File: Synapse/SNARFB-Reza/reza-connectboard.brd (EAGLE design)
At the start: 100 x 80 mm, 6 parts

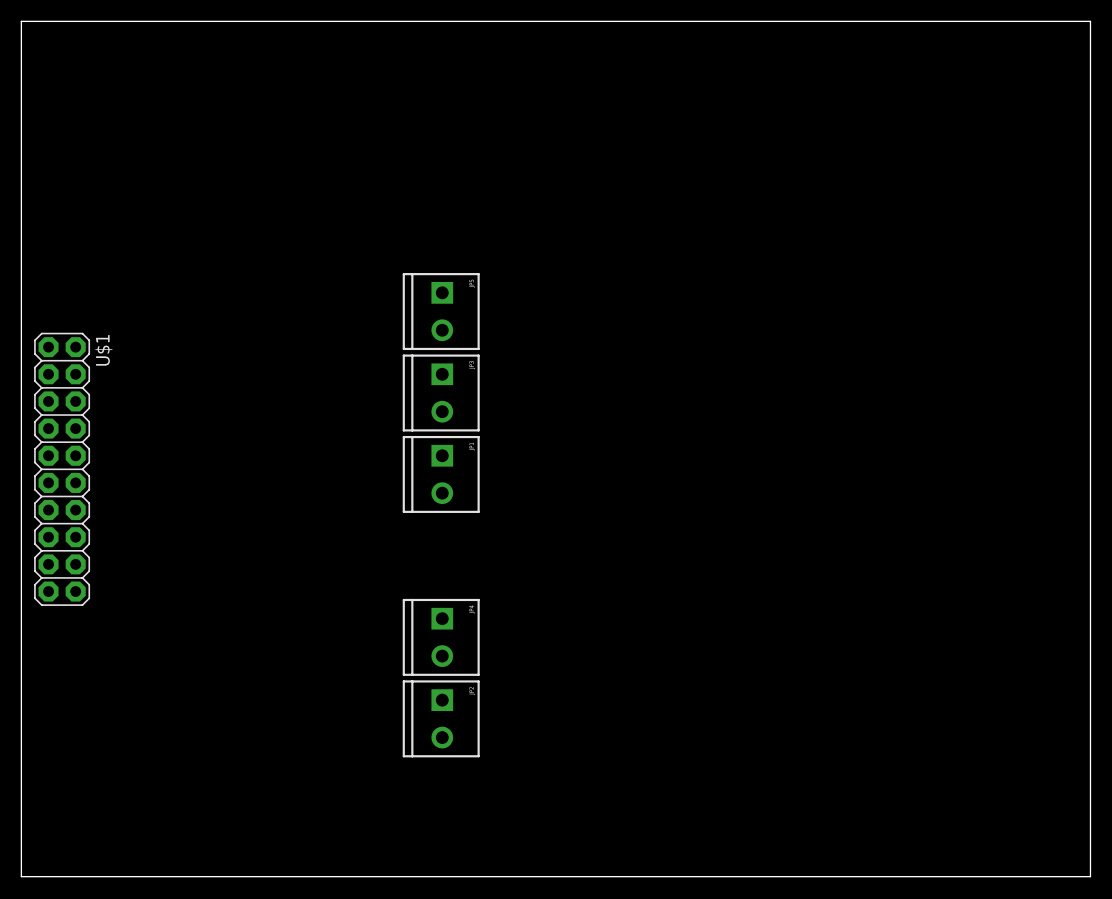
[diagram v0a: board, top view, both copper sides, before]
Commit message: sync
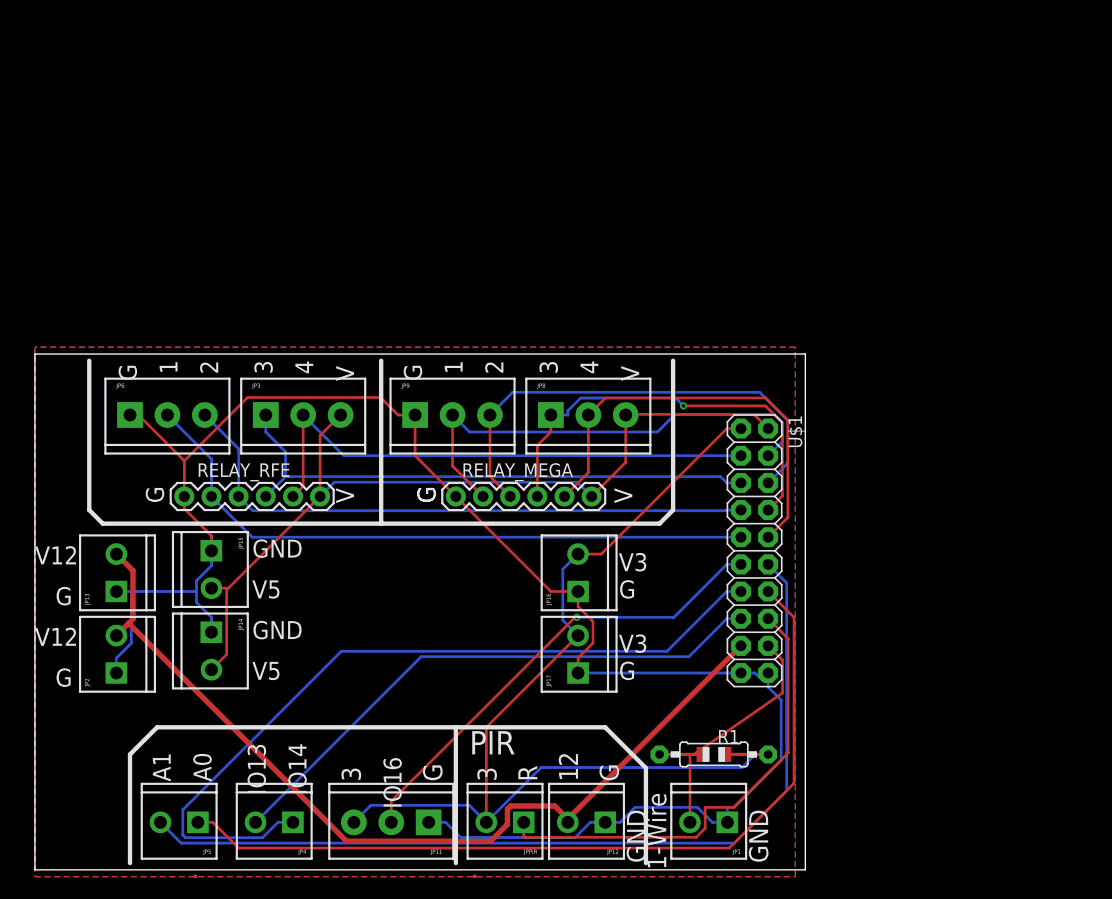
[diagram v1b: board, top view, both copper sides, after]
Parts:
- added JP11, JP6, JP8, JP9: (no value), SparkFun-Connectors:SCREWTERMINAL-3.5MM-3
- added JP12, JP13, JP14, JP15, JP16, JP17, JPPIR: M023.5MM, SparkFun-Connectors:SCREWTERMINAL-3.5MM-2
- added R1: (no value), adafruit:0805-THM
- added RELAY_MEGA, RELAY_RFE: (no value), SparkFun-Connectors:1X06
- added U$2: (no value), 0_jc-custom-eagle6:ENVIOSYS_LOGO2
- JP3: value M023.5MM -> (none); device SparkFun-Connectors:SCREWTERMINAL-3.5MM-2 -> SparkFun-Connectors:SCREWTERMINAL-3.5MM-3
- moved U$1 65.2 mm to (68.6, 30.5)
- moved JP5 54.6 mm to (16.5, 5.08), turned to 180 degrees
- moved JP1 43.4 mm to (66.0, 5.08), turned to 180 degrees
- moved JP2 30.6 mm to (8.89, 19.1), turned to 90 degrees
- moved JP4 23.6 mm to (25.4, 5.08), turned to 180 degrees
- moved JP3 16.9 mm to (22.9, 43.2), turned to 0 degrees
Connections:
- net GND: now also JP1.1, JP11.1, JP12.1, JP13.1, JP14.1, JP15.1, JP16.1, JP17.1, JP2.1, JP6.1, JP9.1, RELAY_MEGA.1, RELAY_RFE.1
- net GPIO13: now also JP4.2
- net GPIO14: now also JP4.1
- net GPIO15: now also JP6.2, RELAY_RFE.2
- net GPIO16: now also JP11.2
- net GPIO2: now also JP3.2, RELAY_RFE.5
- net GPIO5: now also JP3.1, RELAY_RFE.4
- net GPIO6: now also JP6.3, RELAY_RFE.3
- net PC6-D5: now also JPPIR.1
- net PD7-D6: now also JP1.2, R1.2
- net PF0-A5: now also JP9.2, RELAY_MEGA.2
- net PF1-A4: now also JP9.3, RELAY_MEGA.3
- net PF4-A3: now also JP8.1, RELAY_MEGA.4
- net PF5-A2: now also JP8.2, RELAY_MEGA.5
- net PF6-A1: now also JP5.2
- net PF7-A0: now also JP5.1
- net VCC12: now also JP12.2, JP13.2, JP2.2
- net VCC3: now also JP11.3, JP16.2, JP17.2, JPPIR.2, R1.1
- net VCC5: now also JP14.2, JP15.2, JP3.3, JP8.3, RELAY_MEGA.6, RELAY_RFE.6
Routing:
- net GND: track 0.00 -> 163.8 mm
- net VCC3: track 0.00 -> 92.6 mm
- net VCC12: track 0.00 -> 84.3 mm
- net PF6-A1: track 0.00 -> 83.3 mm
- net VCC5: track 0.00 -> 79.7 mm
- net PF7-A0: track 0.00 -> 78.2 mm
- net GPIO14: track 0.00 -> 74.0 mm
- net GPIO15: track 0.00 -> 60.4 mm
- net GPIO6: track 0.00 -> 56.5 mm
- net GPIO13: track 0.00 -> 53.3 mm
- net GPIO5: track 0.00 -> 52.0 mm
- net GPIO2: track 0.00 -> 50.5 mm
- net PF0-A5: track 0.00 -> 45.0 mm
- net PF1-A4: track 0.00 -> 44.9 mm
- net PC6-D5: track 0.00 -> 43.9 mm
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- added copper zone on layer 16, net N$1
- added copper zone on layer 1, net N$2
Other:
- board size 100 x 80 mm -> 72.1 x 48.2 mm
- board text added: "1"
- board text added: "1-Wire"
- board text added: "12"
- board text added: "2"
- board text added: "3"
- board text added: "4"
- board text added: "A0"
- board text added: "A1"
- board text added: "G"
- board text added: "GND"
- board text added: "IO13"
- board text added: "IO14"
- board text added: "IO16"
- board text added: "PIR"
- board text added: "R"
- board text added: "V"
- board text added: "V12"
- board text added: "V3"
- board text added: "V5"
